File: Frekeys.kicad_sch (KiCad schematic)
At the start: 12 parts, among them J1 AudioPlug3, SW1 RotaryEncoder_Switch, U1 CR2013-MI2120, U2 ESP32-S3-DevKitC, U3 74HC165, U4 74HC165

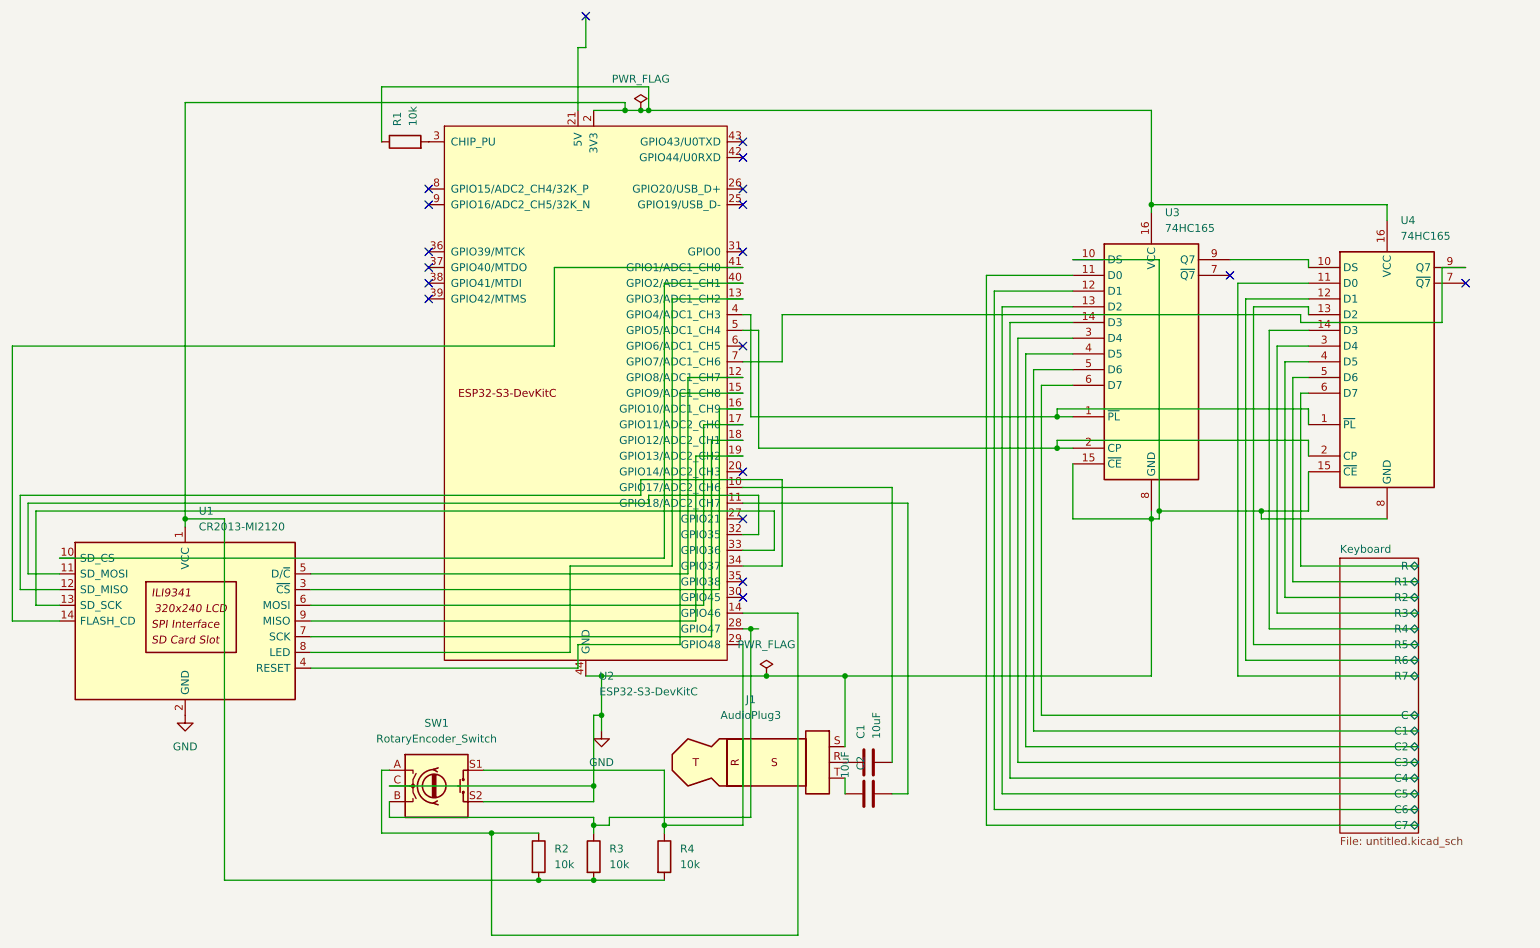
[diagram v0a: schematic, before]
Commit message: Making.. 2
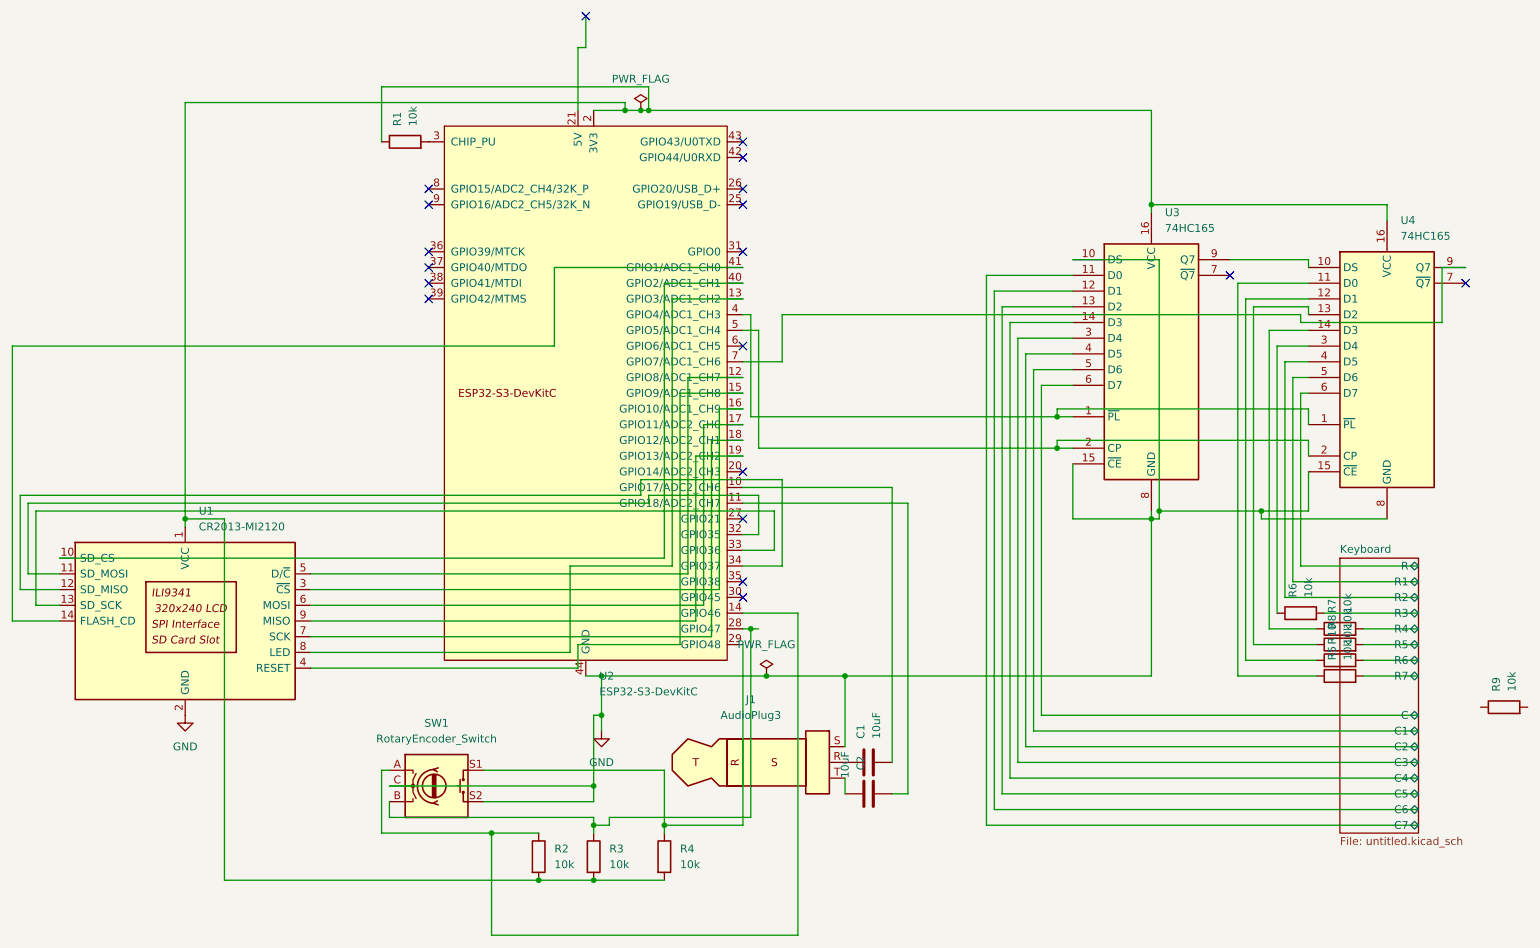
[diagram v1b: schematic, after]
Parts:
- added R10, R5, R6, R7, R8, R9: 10k, Resistor_SMD:R_0805_2012Metric, symbol Device:R
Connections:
- net Keyboard/R3: now also R6.2; no longer U4.3 (D4)
- net Keyboard/R4: now also R7.2; no longer U4.14 (D3)
- net Keyboard/R5: now also R8.2; no longer U4.13 (D2)
- net Keyboard/R6: now also R10.2; no longer U4.12 (D1)
- net Keyboard/R7: now also R5.2; no longer U4.11 (D0)
- new net: R5.1, U4.11 (D0)
- new net: R8.1, U4.13 (D2)
- new net: R7.1, U4.14 (D3)
- new net: R10.1, U4.12 (D1)
- new net: R6.1, U4.3 (D4)
